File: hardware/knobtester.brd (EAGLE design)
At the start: 30.5 x 40.3 mm, 8 parts

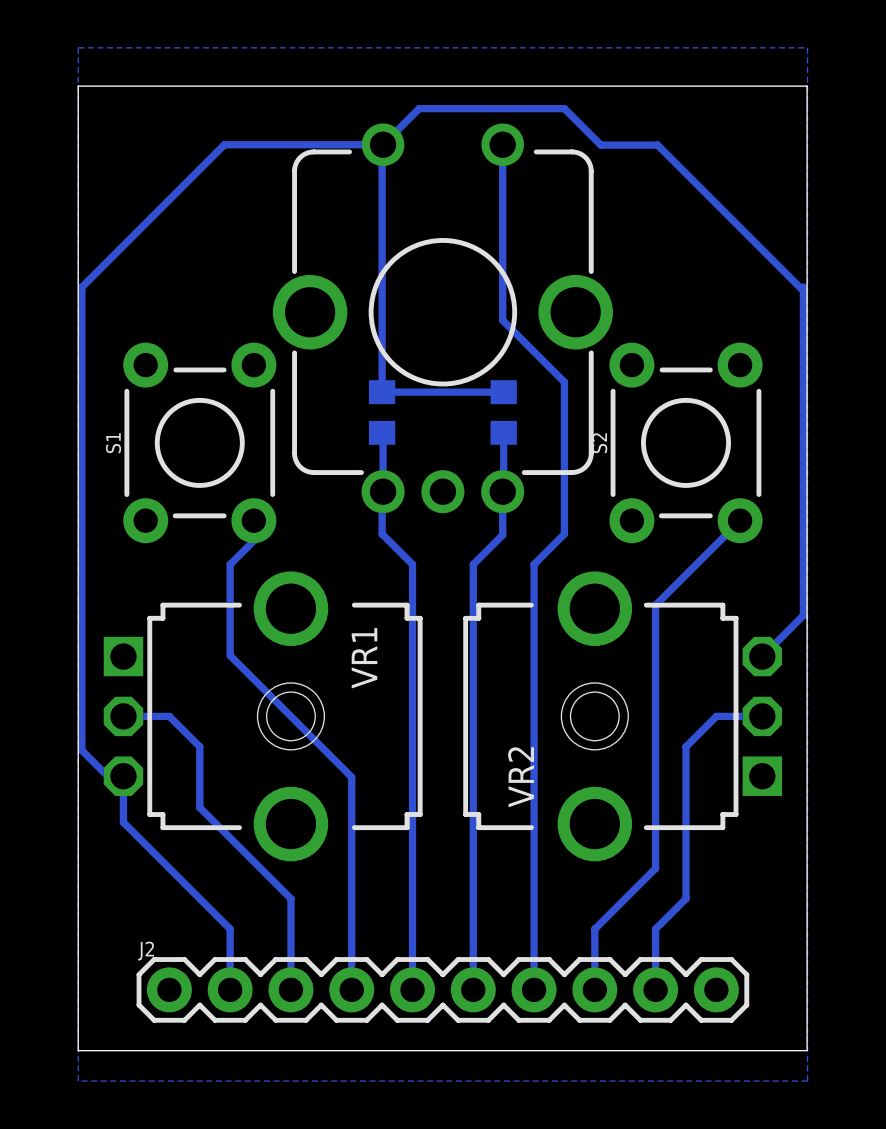
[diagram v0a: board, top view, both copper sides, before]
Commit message: updates
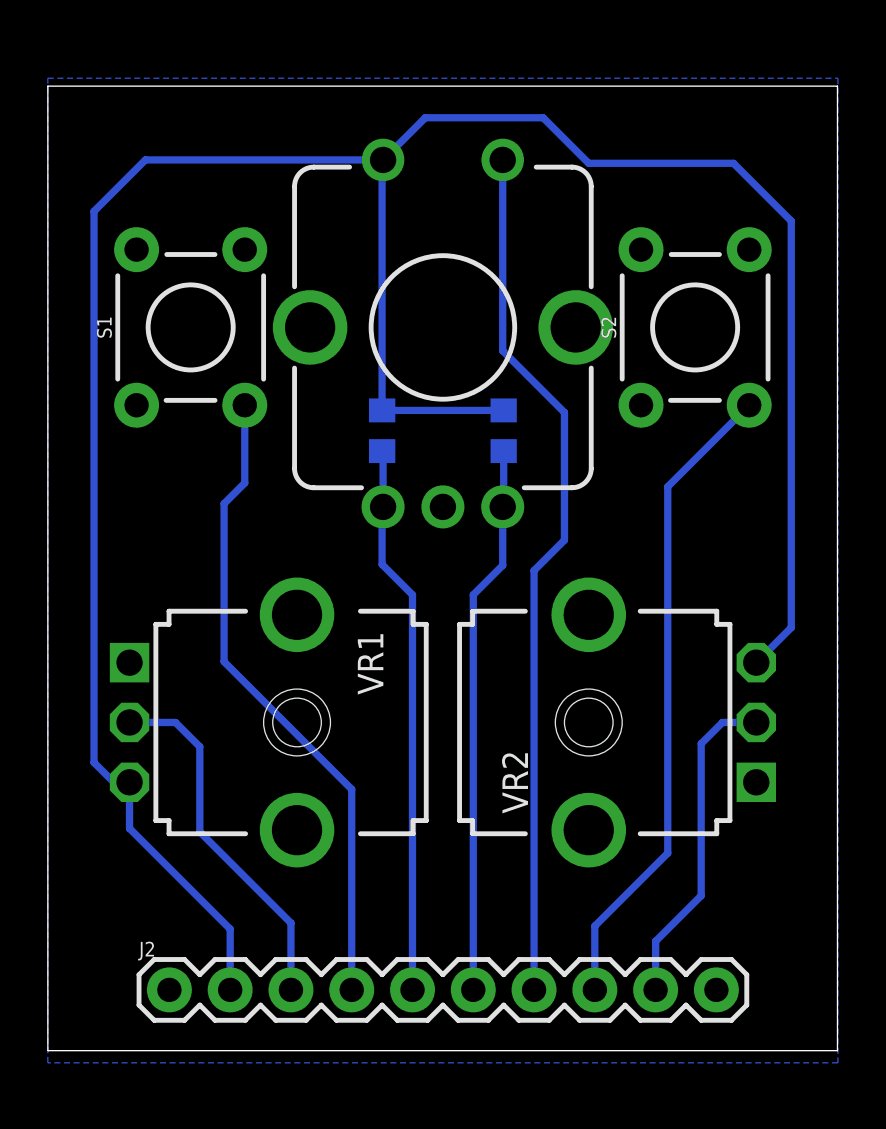
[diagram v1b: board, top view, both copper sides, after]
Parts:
- moved S1 4.84 mm to (4.70, 30.2)
- moved S2 4.84 mm to (25.8, 30.2)
- moved R16 0.76 mm to (12.7, 25.9)
- moved R17 0.76 mm to (17.8, 25.9)
- moved U$1 0.64 mm to (15.2, 30.2)
- moved VR2 0.36 mm to (21.3, 13.7)
- moved VR1 0.36 mm to (9.14, 13.7)
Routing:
- net SW2: track 22.1 -> 27.1 mm
- net SW1: track 22.1 -> 27.0 mm
- net +3V3: track 100.3 -> 102.5 mm
- net ENCB: track 23.8 -> 23.0 mm
- net ENCA: track 23.8 -> 23.1 mm
- net KNOB2: track 14.4 -> 13.7 mm
- net ENCSW: track 36.9 -> 36.3 mm
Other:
- board size 30.5 x 40.3 mm -> 33 x 40.3 mm
